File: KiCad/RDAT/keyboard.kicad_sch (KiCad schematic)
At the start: 231 parts, among them J1 Conn_01x02, J2 Conn_01x02, U1 W25Q128JVS, U2 SC091413, X1 ABM8-272-T3

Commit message: Wrong footprint for keyswitches, creating save point
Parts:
- S1, S10, S100, S101, S102, S103, S11, S12, S13, S14, S15, S16, S17, S18, S19, S2, S20, S21, S22, S23, S24, S25, S26, S27, S28, S29, S3, S30, S31, S32, S33, S34, S35, S36, S37, S38, S39, S4, S40, S41, S42, S43, S44, S45, S46, S47, S48, S49, S5, S50, S51, S52, S53, S54, S55, S56, S57, S58, S59, S6, S60, S61, S62, S63, S64, S65, S66, S67, S68, S69, S7, S70, S71, S72, S73, S74, S75, S76, S77, S78, S79, S8, S80, S81, S82, S83, S84, S85, S86, S87, S88, S89, S9, S90, S91, S92, S93, S94, S95, S96, S97, S98, S99: footprint footprints:SW_PG151101S11 -> keyswitches:Kailh_socket_PG1350_optional

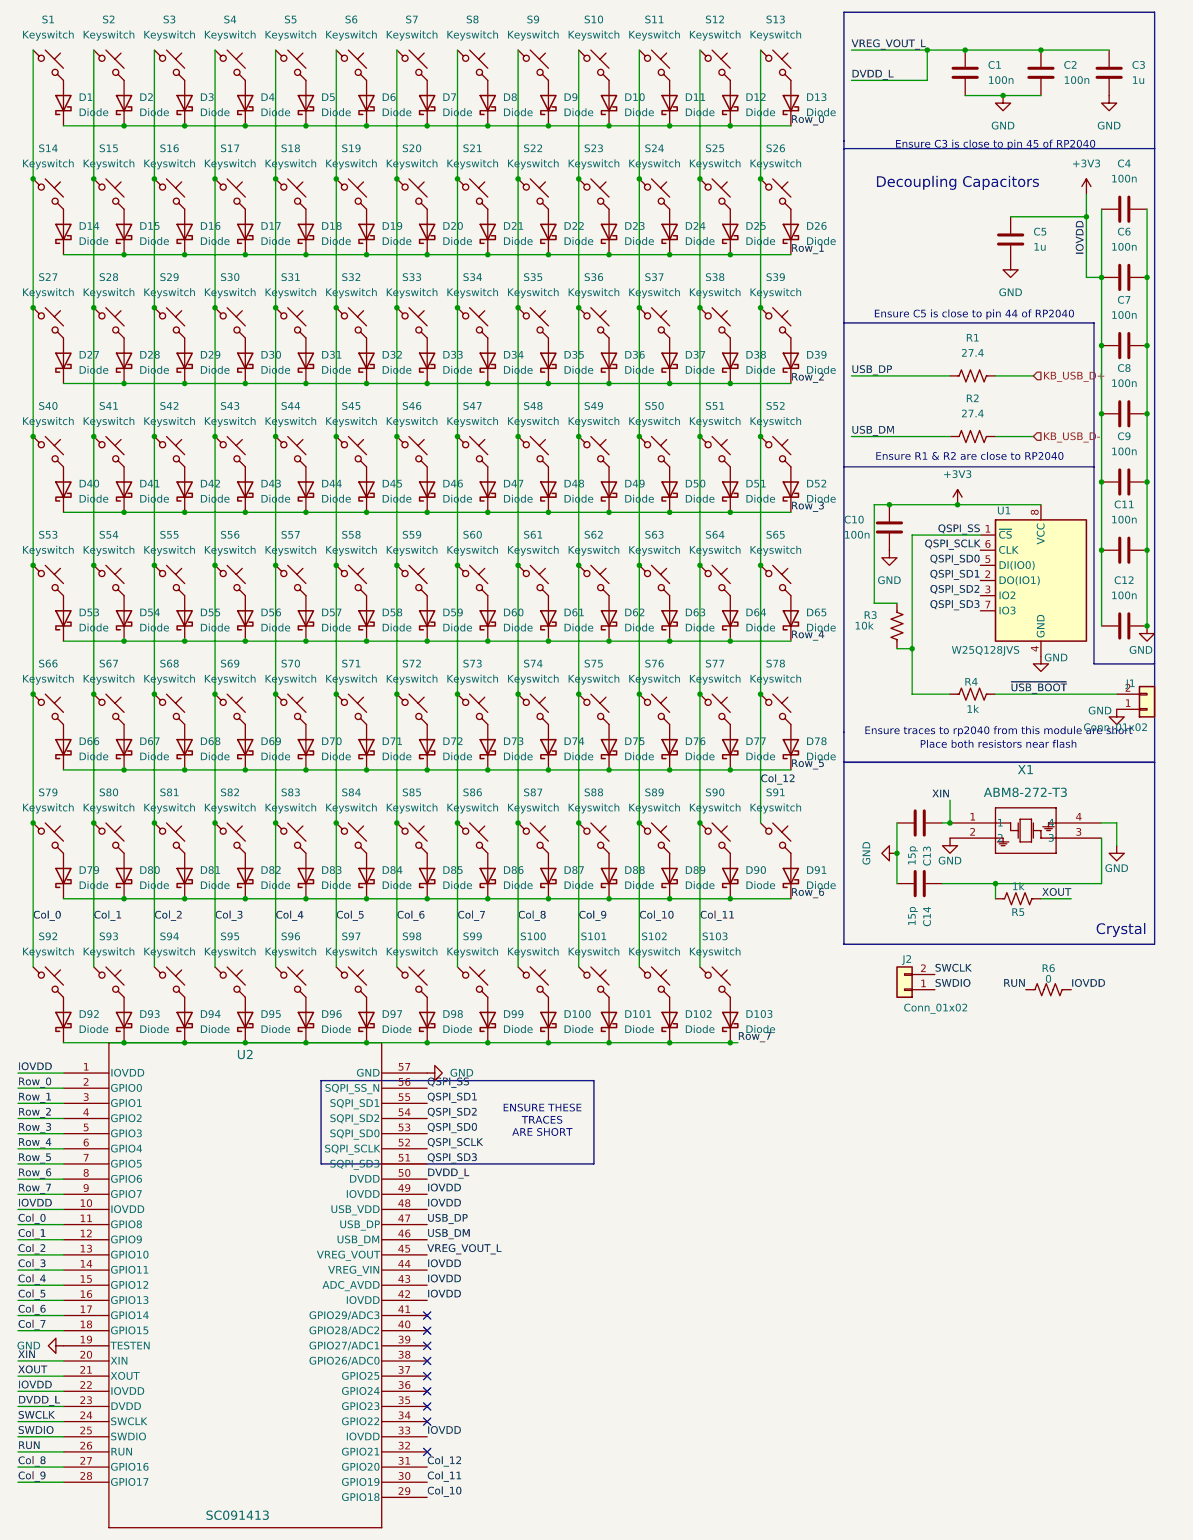
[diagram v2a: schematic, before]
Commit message: 2x checing of bom on JLCPCB
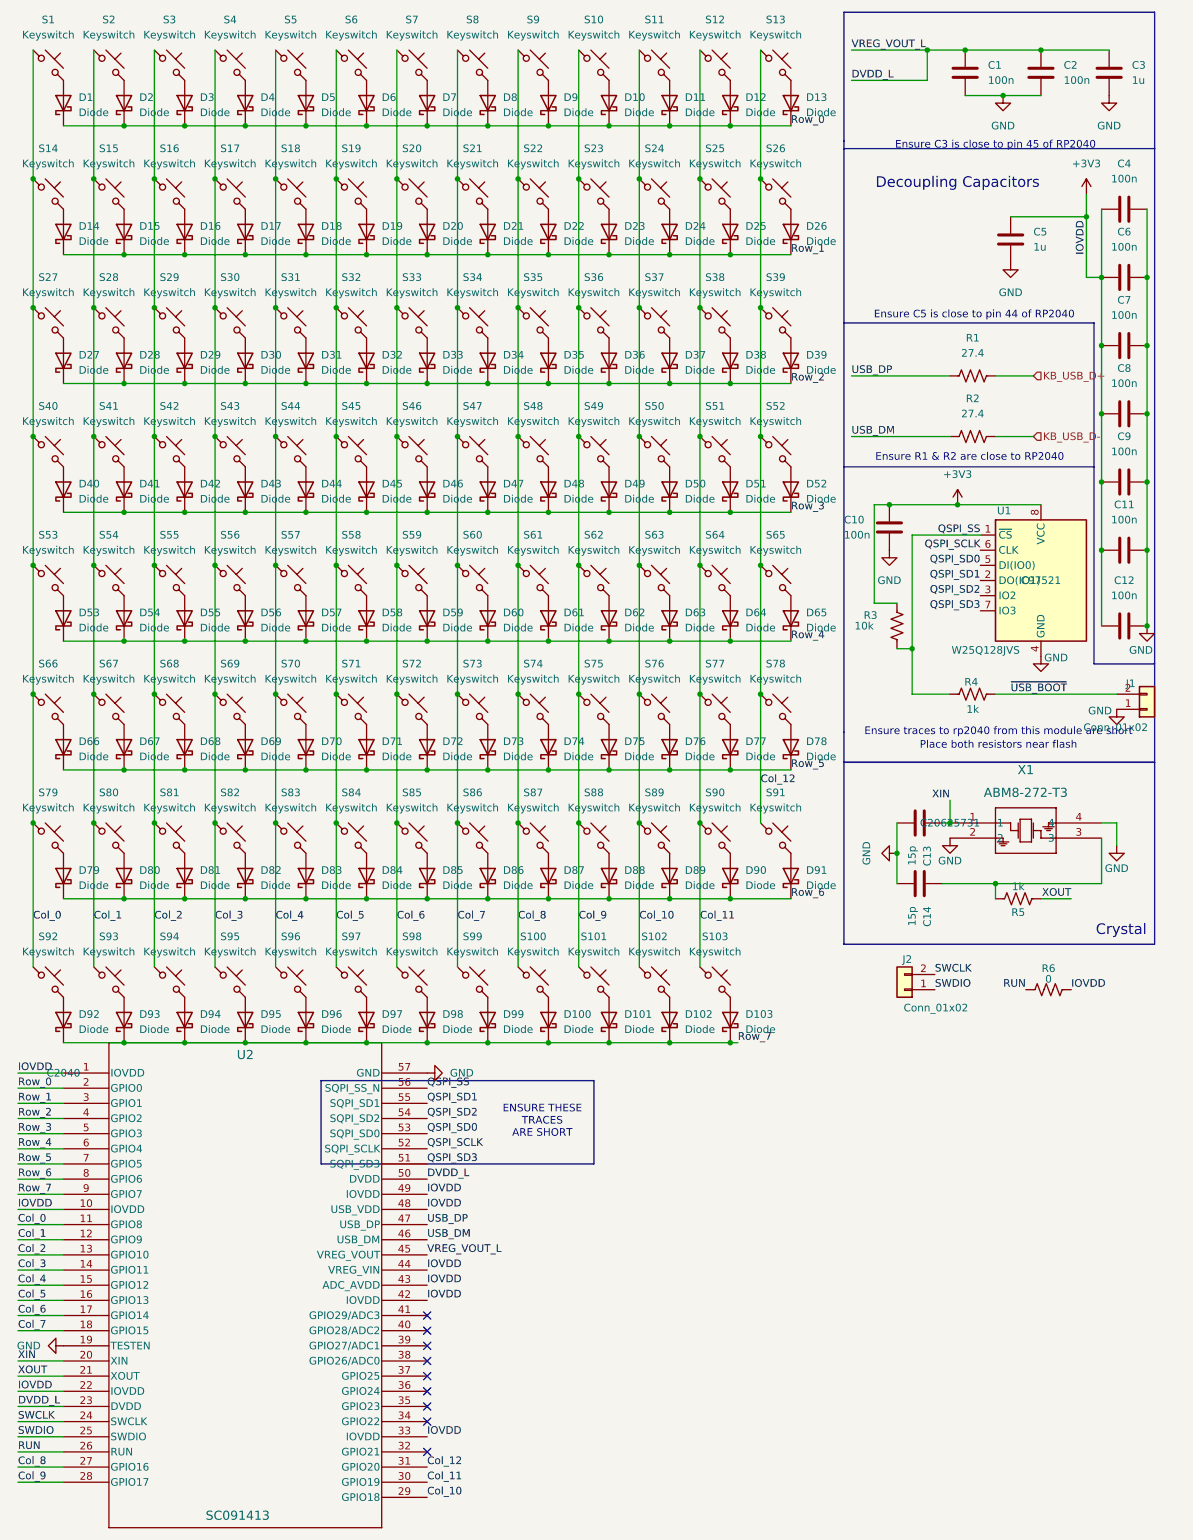
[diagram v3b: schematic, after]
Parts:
- U1: JLCPCB_PART_NUMBER (none) -> C97521
- U2: JLCPCB_PART_NUMBER (none) -> C2040
- X1: JLCPCB_LINK https://jlcpcb.com/parts/componentSearch?searchTxt=ABM8-272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 -> https://jlcpcb.com/partdetail/AbraconLlc-ABM8_272T3/C206257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; JLCPCB_PART_NUMBER (none) -> C20625731
